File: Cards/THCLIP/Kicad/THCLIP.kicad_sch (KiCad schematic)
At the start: 12 parts, among them J2 Conn_01x03_Pin, J3 Conn_01x05_Pin, K1 Relay_SPDT, U1 RS3K-2424S/H3

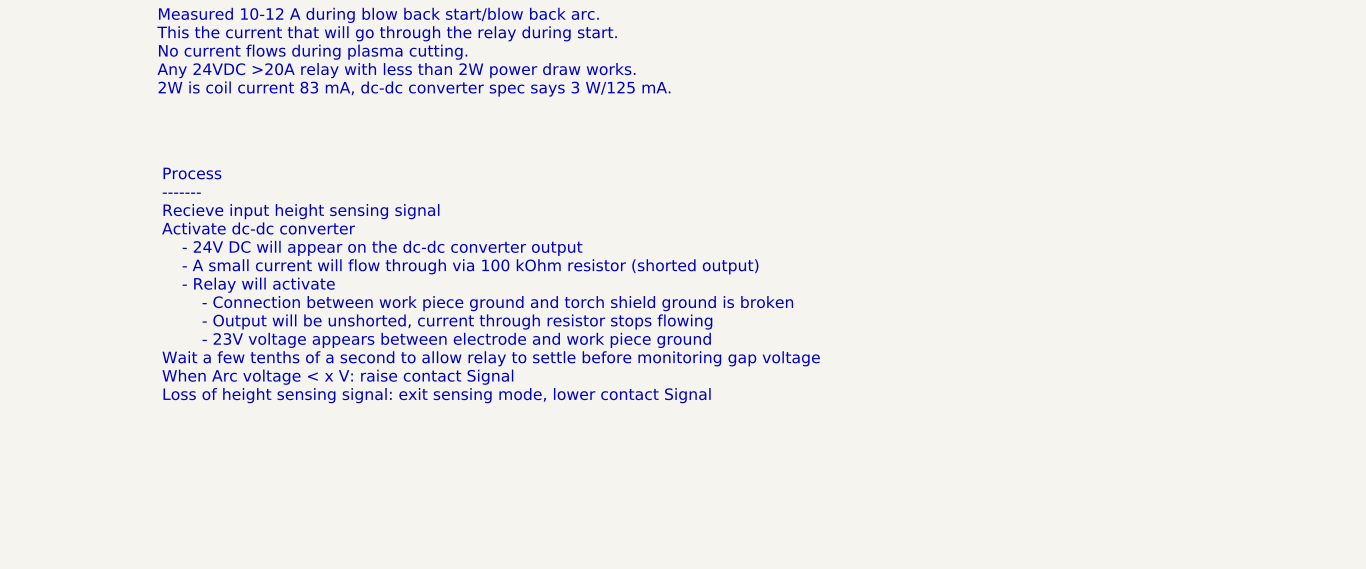
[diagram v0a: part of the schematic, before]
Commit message: updated process description more
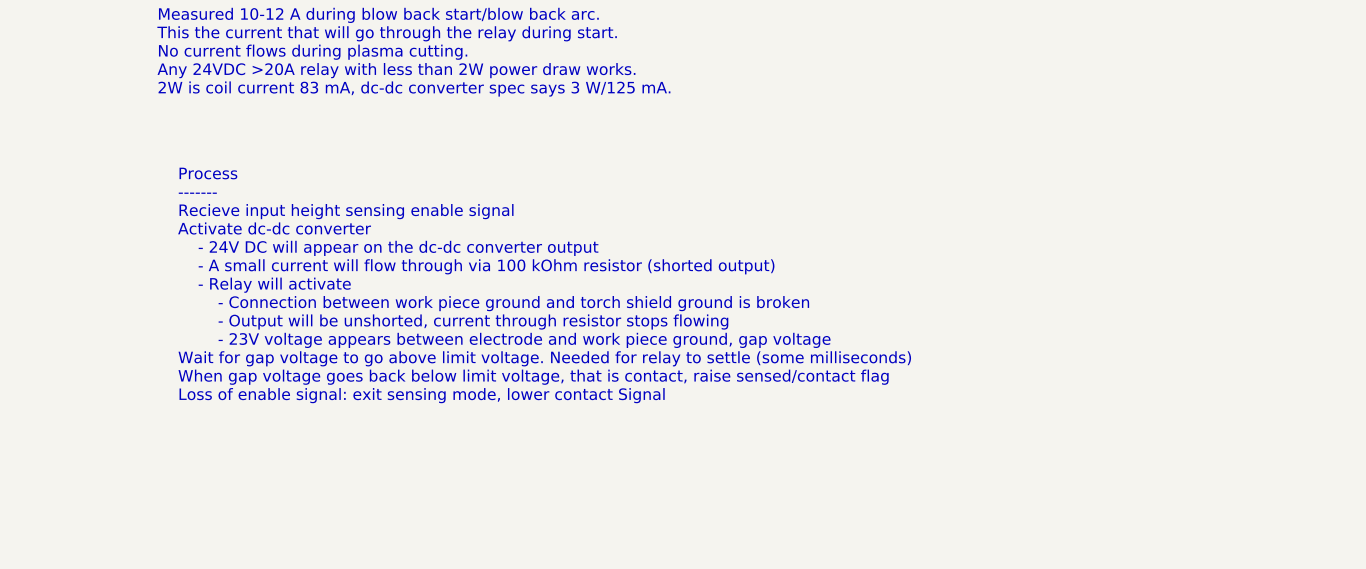
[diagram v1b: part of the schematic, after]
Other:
- note added: "Process ------- Recieve input height sensing enable signal Activate dc-dc converter - 24V DC will appear on the dc-dc converter output - A small current will flow through via 100 kOhm resistor (shorted output) - Relay will activate - Connection between work piece ground and torch shield ground is broken - Output will be unshorted, current through resistor stops flowing - 23V voltage appears betwe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"
- note removed: "Process ------- Recieve input height sensing signal Activate dc-dc converter - 24V DC will appear on the dc-dc converter output - A small current will flow through via 100 kOhm resistor (shorted output) - Relay will activate - Connection between work piece ground and torch shield ground is broken - Output will be unshorted, current through resistor stops flowing - 23V voltage appears between elec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"
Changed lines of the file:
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@@
 		)
 	)
-	(text "Process\n-------\nRecieve input height sensing signal\nActivate dc-dc converter\n	- 24V DC will appear on the dc-dc converter output\n	- A small current will flow through via 100 kOhm resistor (shorted output)\n	- Relay will activate\n		- Connection between work piece ground and torch shield ground is broken\n		- Output will be unshorted, current through resistor stops flowing\n		- 23V voltage appears between electrode and work piece ground\nWait a few tenths of a second to allow relay to settle before monitoring gap voltage\nWhen Arc voltage < x V: raise contact Signal\nLoss of height sensing signal: exit sensing mode, lower contact Signal\n\n"
+	(text "Process\n-------\nRecieve input height sensing enable signal\nActivate dc-dc converter\n	- 24V DC will appear on the dc-dc converter output\n	- A small current will flow through via 100 kOhm resistor (shorted output)\n	- Relay will activate\n		- Connection between work piece ground and torch shield ground is broken\n		- Output will be unshorted, current through resistor stops flowing\n		- 23V voltage appears between electrode and work piece ground, gap voltage\nWait for gap voltage to go above limit voltage. Needed for relay to settle (some milliseconds)\nWhen gap voltage goes back below limit voltage, that is contact, raise sensed/contact flag\nLoss of enable signal: exit sensing mode, lower contact Signal\n\n"
 		(exclude_from_sim no)
-		(at 88.646 131.826 0)
+		(at 90.424 131.826 0)
 		(effects
 			(font
